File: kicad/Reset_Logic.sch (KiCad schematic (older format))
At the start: 9 parts

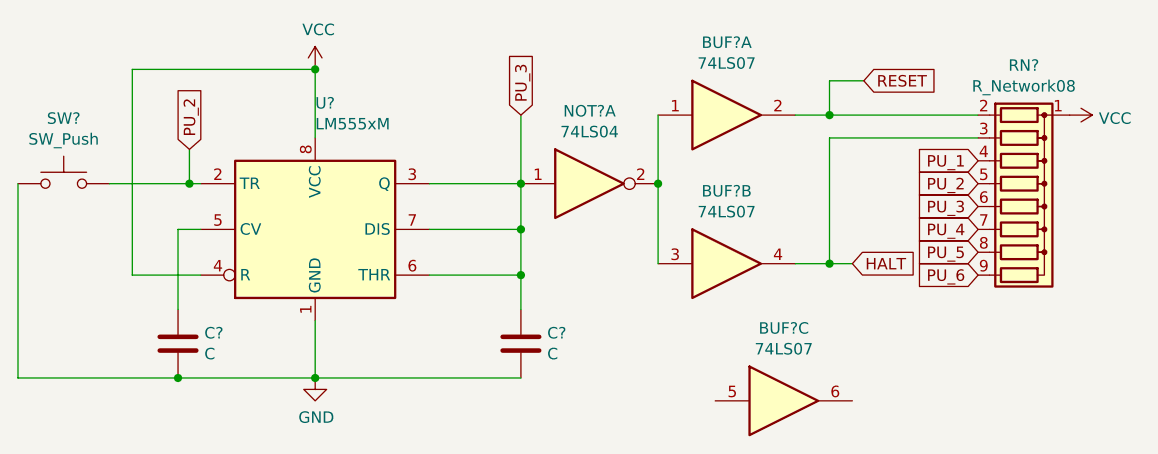
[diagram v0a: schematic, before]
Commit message: Almost ready to route the PCB fully
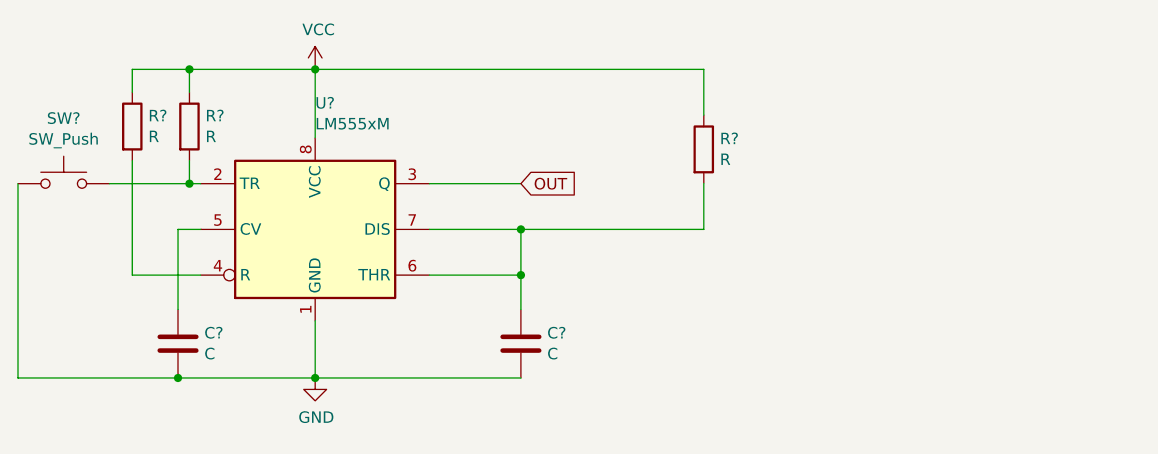
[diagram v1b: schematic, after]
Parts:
- removed BUF? (x3): 74LS07, symbol 74xx:74LS07
- removed NOT?: 74LS04, symbol 74xx:74LS04
- removed RN?: R_Network08, Resistor_THT:R_Array_SIP9, symbol Device:R_Network08
- added R? (x3): R, symbol Device:R
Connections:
- net VCC: now also R?.1, R?.1, R?.1; no longer U?.4 (R)
- net PU_2: no longer names the net of SW?.2, U?.2 (TR)
- net PU_2: now also R?.2
- net PU_3: no longer names the net of C?.1, U?.6 (THR), U?.7 (DIS)
- net PU_3: now also R?.2; no longer U?.3 (Q)
- new net: R?.2, U?.4 (R)
- new net OUT: U?.3 (Q)
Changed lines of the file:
@@
 $Descr A4 11693 8268
 encoding utf-8
-Sheet 3 2
+Sheet 1 1
 Title ""
 Date ""
@@
 Comment4 ""
 $EndDescr
-$Comp
-L 74xx:74LS07 BUF?
-U 1 1 61148731
-P 6600 3600
-F 0 "BUF?" H 6600 3917 50  0000 C CNN
-F 1 "74LS07" H 6600 3826 50  0000 C CNN
-F 2 "" H 6600 3600 50  0001 C CNN
-F 3 "www.ti.com/lit/ds/symlink/sn74ls07.pdf" H 6600 3600 50  0001 C CNN
-	1    6600 3600
-	1    0    0    -1
-$EndComp
-$Comp
-L 74xx:74LS07 BUF?
-U 2 1 61148737
-P 6600 4250
-F 0 "BUF?" H 6600 4567 50  0000 C CNN
-F 1 "74LS07" H 6600 4476 50  0000 C CNN
-F 2 "" H 6600 4250 50  0001 C CNN
-F 3 "www.ti.com/lit/ds/symlink/sn74ls07.pdf" H 6600 4250 50  0001 C CNN
-	2    6600 4250
-	1    0    0    -1
-$EndComp
-$Comp
-L 74xx:74LS07 BUF?
-U 3 1 6114873D
-P 6850 4850
-F 0 "BUF?" H 6850 5167 50  0000 C CNN
-F 1 "74LS07" H 6850 5076 50  0000 C CNN
-F 2 "" H 6850 4850 50  0001 C CNN
-F 3 "www.ti.com/lit/ds/symlink/sn74ls07.pdf" H 6850 4850 50  0001 C CNN
-	3    6850 4850
-	1    0    0    -1
-$EndComp
-Wire Wire Line
-	6900 3600 7050 3600
-Wire Wire Line
-	6900 4250 7050 4250
-Wire Wire Line
-	7050 3600 7050 3450
-Wire Wire Line
-	7050 3450 7200 3450
-Text GLabel 7200 3450 2    50   Input ~ 0
-RESET
-Text GLabel 7150 4250 2    50   Input ~ 0
-HALT
-Wire Wire Line
-	7050 4250 7150 4250
-Connection ~ 7050 4250
 $Comp
 L Timer:LM555xM U?
@@
 	5300 3900 5700 3900
 Wire Wire Line
-	5700 3900 5700 3600
-Wire Wire Line
 	5300 4100 5700 4100
 Wire Wire Line
-	5700 4100 5700 3900
-Connection ~ 5700 3900
-Wire Wire Line
 	5300 4300 5700 4300
-Wire Wire Line
-	5700 4300 5700 4100
-Connection ~ 5700 4100
 $Comp
 L Device:C C?
@@
 Wire Wire Line
 	4800 4750 5700 4750
-$Comp
-L 74xx:74LS04 NOT?
-U 1 1 6114877B
-P 6000 3900
-F 0 "NOT?" H 6000 4217 50  0000 C CNN
-F 1 "74LS04" H 6000 4126 50  0000 C CNN
-F 2 "" H 6000 3900 50  0001 C CNN
-F 3 "http://www.ti.com/lit/gpn/sn74LS04" H 6000 3900 50  0001 C CNN
-	1    6000 3900
-	1    0    0    -1
-$EndComp
-Connection ~ 5700 4300
-Wire Wire Line
-	5700 4300 5700 4450
-Wire Wire Line
-	6300 3600 6300 3900
-Connection ~ 6300 3900
-Wire Wire Line
-	6300 3900 6300 4250
 Connection ~ 4200 4750
 Wire Wire Line
@@
 	4200 4750 4800 4750
 Wire Wire Line
-	7050 4250 7050 3700
+	4800 3400 4800 3700
+Connection ~ 4800 3400
 $Comp
-L power:VCC #PWR?
-U 1 1 6114878D
-P 8100 3600
-F 0 "#PWR?" H 8100 3450 50  0001 C CNN
-F 1 "VCC" V 8115 3728 50  0000 L CNN
-F 2 "" H 8100 3600 50  0001 C CNN
-F 3 "" H 8100 3600 50  0001 C CNN
-	1    8100 3600
-	0    1    1    0
+L Device:R R?
+U 1 1 616A3CF3
+P 4000 3650
+F 0 "R?" H 4070 3696 50  0000 L CNN
+F 1 "R" H 4070 3605 50  0000 L CNN
+F 2 "" V 3930 3650 50  0001 C CNN
+F 3 "~" H 4000 3650 50  0001 C CNN
+	1    4000 3650
+	1    0    0    -1
 $EndComp
-Connection ~ 7050 3600
-Text GLabel 7700 3800 0    50   Input ~ 0
-PU_1
-Text GLabel 7700 3900 0    50   Input ~ 0
-PU_2
-Text GLabel 7700 4000 0    50   Input ~ 0
-PU_3
-Text GLabel 4250 3750 1    50   Input ~ 0
-PU_2
-Text GLabel 5700 3600 1    50   Input ~ 0
-PU_3
-Wire Wire Line
-	4000 3400 4800 3400
 $Comp
-L Device:R_Network08 RN?
-U 1 1 6114879A
-P 7900 4000
-F 0 "RN?" V 7283 4000 50  0000 C CNN
-F 1 "R_Network08" V 7374 4000 50  0000 C CNN
-F 2 "Resistor_THT:R_Array_SIP9" V 8375 4000 50  0001 C CNN
-F 3 "http://www.vishay.com/docs/31509/csc.pdf" H 7900 4000 50  0001 C CNN
-	1    7900 4000
-	0    1    1    0
+L Device:R R?
+U 1 1 616A4A7C
+P 4250 3650
+F 0 "R?" H 4320 3696 50  0000 L CNN
+F 1 "R" H 4320 3605 50  0000 L CNN
+F 2 "" V 4180 3650 50  0001 C CNN
+F 3 "~" H 4250 3650 50  0001 C CNN
+	1    4250 3650
+	1    0    0    -1
 $EndComp
 Wire Wire Line
-	7050 3700 7700 3700
+	4000 3400 4000 3500
 Wire Wire Line
-	7050 3600 7700 3600
-Text GLabel 7700 4100 0    50   Input ~ 0
-PU_4
-Text GLabel 7700 4200 0    50   Input ~ 0
-PU_5
-Text GLabel 7700 4300 0    50   Input ~ 0
-PU_6
+	5700 4100 5700 4300
+Wire Wire Line
+	5700 4300 5700 4450
+Connection ~ 5700 4300
+Wire Wire Line
+	4800 3400 6500 3400
+Wire Wire Line
+	6500 4100 5700 4100
+Connection ~ 5700 4100
+$Comp
+L Device:R R?
+U 1 1 616A6B77
+P 6500 3750
+F 0 "R?" H 6570 3796 50  0000 L CNN
+F 1 "R" H 6570 3705 50  0000 L CNN
+F 2 "" V 6430 3750 50  0001 C CNN
+F 3 "~" H 6500 3750 50  0001 C CNN
+	1    6500 3750
+	1    0    0    -1
+$EndComp
+Wire Wire Line
+	6500 3600 6500 3400
+Wire Wire Line
+	6500 3900 6500 4100
+Wire Wire Line
+	4000 3800 4000 4300
+Wire Wire Line
+	4000 3400 4250 3400
 Wire Wire Line
 	3900 3900 4250 3900
 Wire Wire Line
-	4250 3900 4250 3750
+	4250 3900 4250 3800
 Connection ~ 4250 3900
 Wire Wire Line
 	4250 3900 4300 3900
 Wire Wire Line
-	4000 4300 4000 3400
+	4250 3500 4250 3400
+Connection ~ 4250 3400
 Wire Wire Line
-	4800 3400 4800 3700
-Connection ~ 4800 3400
+	4250 3400 4800 3400
+Text GLabel 5700 3900 2    50   Input ~ 0
+OUT
 $EndSCHEMATC
